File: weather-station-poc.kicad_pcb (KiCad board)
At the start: 4 copper layers, 160 x 80 mm, 135 parts, among them IC1 632723100011, IC2 TCPP01-M12, IC3 USBLC6-2SC6, IC4 BME690, IC5 S2-LPQTR, IC6 BALF-SPI2-01D3, IC7 STSAFA110S8OCD03, J1 Conn_ARM_JTAG_SWD_10, J2 61300311121, J3 61300311121, J4 61300511121, J5 61300311121, J6 687140149022, J7 687110183622, Q1 STL11N3LLH6, U1 STM32U5G9ZJTxQ, U2 BME280, U3 BMP581, Y1 NX2016SA-16MHZ-EXS00A-CS07826, Y2 NX2012SA-32.768K-STD-MUB-1, Y3 NX1612SA-50M-EXS00A-CS08403

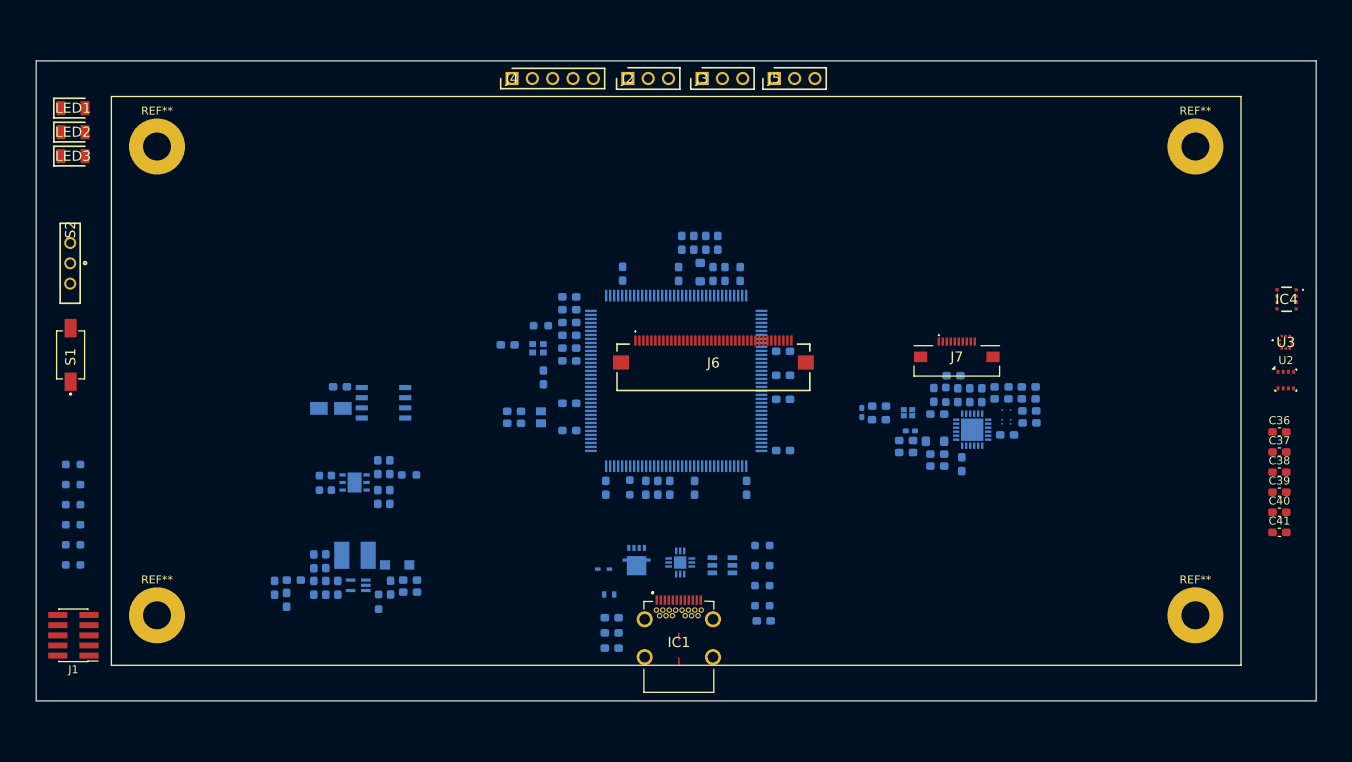
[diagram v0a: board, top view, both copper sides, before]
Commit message: All components placed on PCB
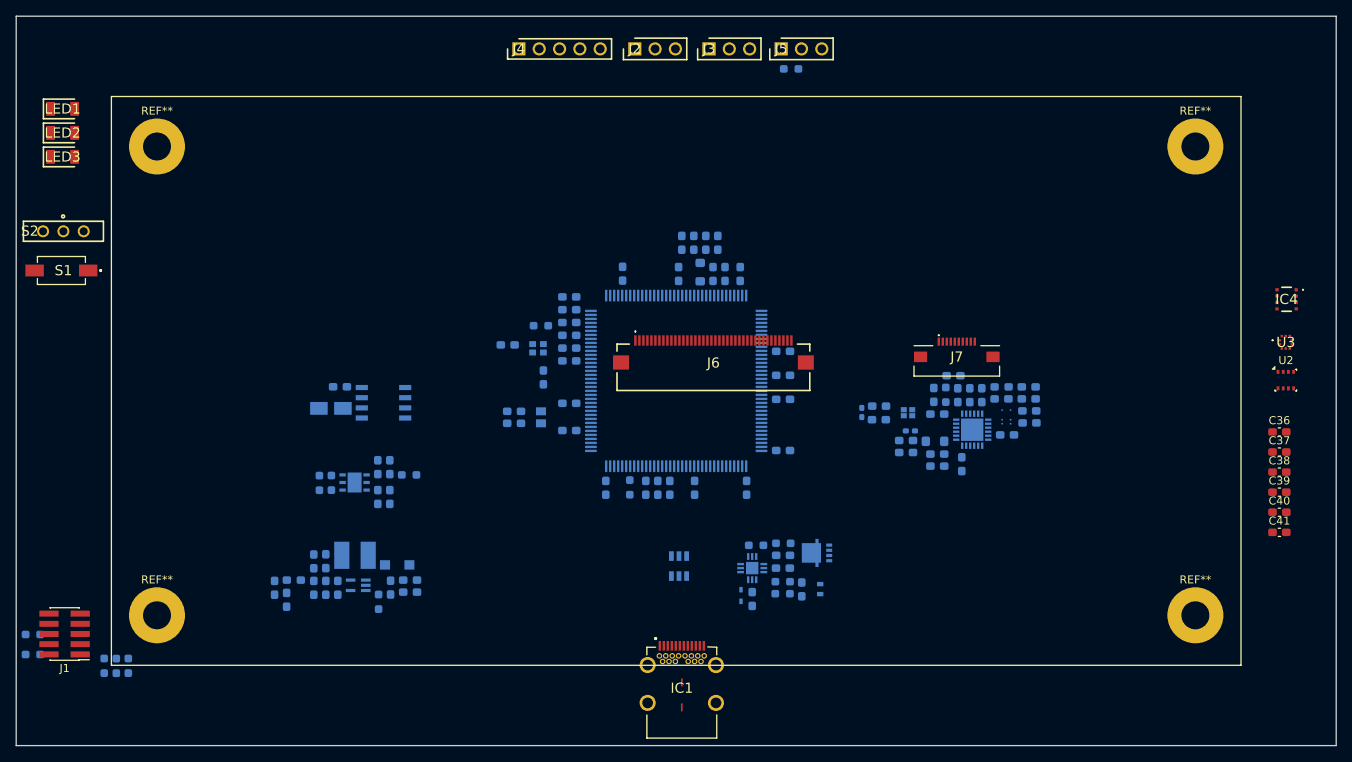
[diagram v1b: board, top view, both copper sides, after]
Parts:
- moved R17 102.5 mm to (160.1, 52.5)
- moved D1 26.4 mm to (163.7, 117.5), turned to 90 degrees
- moved C2 24.9 mm to (161.4, 117.6), turned to -90 degrees
- moved C3 23.5 mm to (159.1, 113.3)
- moved Q1 22.6 mm to (163.3, 113.0), turned to -90 degrees
- moved R16 19.4 mm to (65.3, 123.2), turned to 180 degrees
- moved R15 19.4 mm to (65.3, 125.7), turned to 180 degrees
- moved R14 18.9 mm to (77.2, 127.1), turned to -90 degrees
- moved C4 17.7 mm to (155.2, 118.8), turned to -90 degrees
- moved D2 17.5 mm to (153.8, 118.3), turned to -90 degrees
- moved R13 16.1 mm to (75.7, 127.1), turned to -90 degrees
- moved R12 13.2 mm to (74.2, 127.1), turned to -90 degrees
- moved S1 10.6 mm to (68.8, 77.7), turned to 180 degrees
- moved IC2 9.03 mm to (155.2, 114.9), turned to -90 degrees
- moved S2 8.05 mm to (71.1, 70.8), turned to 0 degrees
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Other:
- board size 160 x 80 mm -> 165 x 91.2 mm
